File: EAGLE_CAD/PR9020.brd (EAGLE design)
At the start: 70 x 70 mm, 73 parts

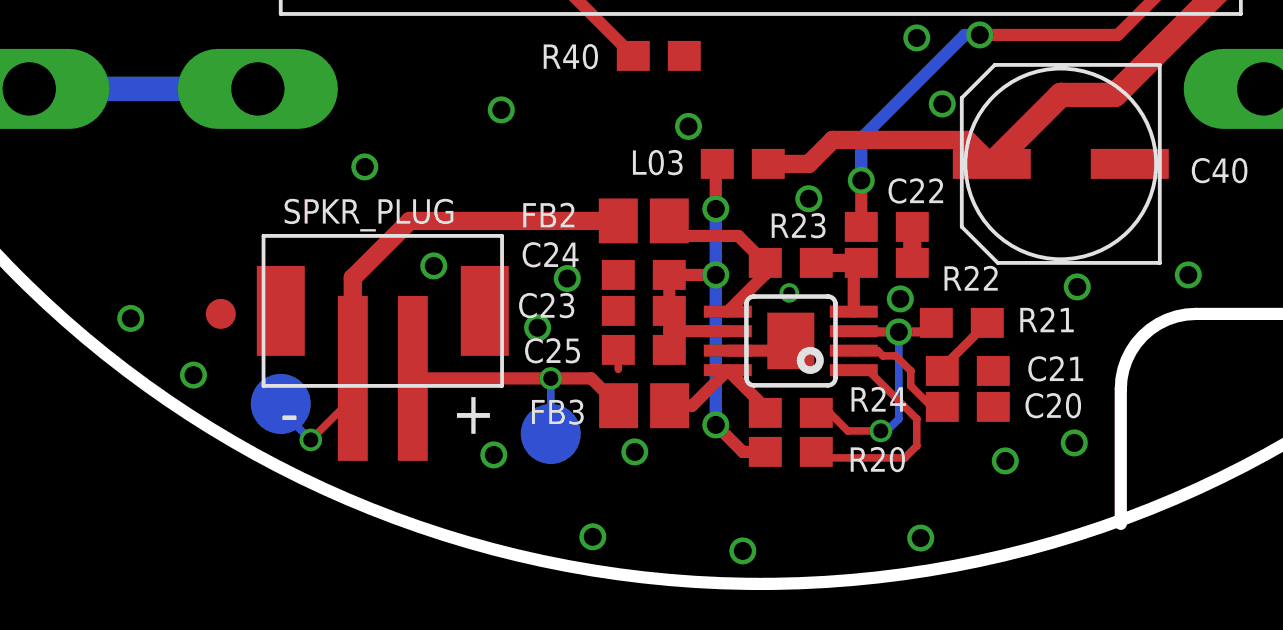
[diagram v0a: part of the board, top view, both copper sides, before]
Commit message: PR9020 Gerbers
PR9020 Gerbers, organized folders
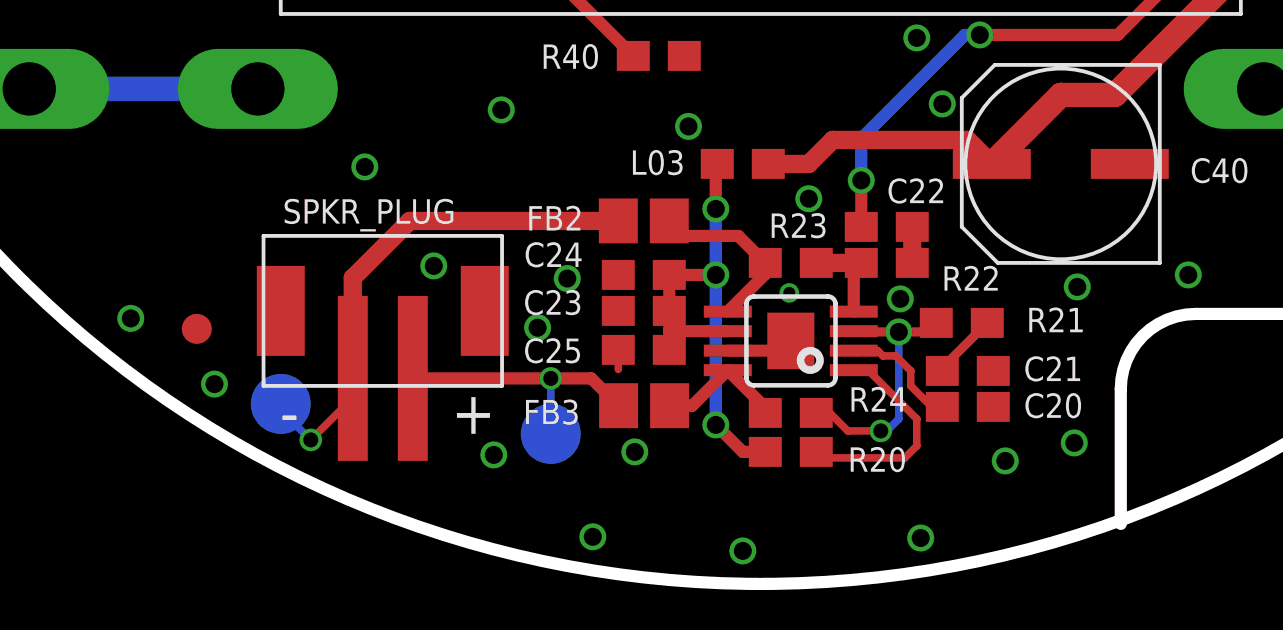
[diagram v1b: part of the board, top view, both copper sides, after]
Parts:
- moved MARK1 0.94 mm to (16.2, 8.50)
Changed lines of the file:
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@@
 <rectangle x1="35.3949" y1="12.6365" x2="35.4711" y2="12.6619" layer="26" rot="R180"/>
 <rectangle x1="35.4203" y1="12.6619" x2="35.5981" y2="12.6873" layer="26" rot="R180"/>
-<text x="64" y="35" size="0.8128" layer="26" font="vector" ratio="18" rot="MR270" align="center">PR9020
+<text x="64" y="35" size="0.8128" layer="26" font="vector" ratio="22" rot="MR270" align="center">PR9020
 Born + tuned in Brooklyn
 http://thepublicrad.io</text>
@@
 </element>
 <element name="R21" library="PR_Parts_Library" package="0603_CPL" value="12K" x="41.7" y="8.7" smashed="yes" rot="R180">
-<attribute name="NAME" x="43.551" y="8.389" size="0.8128" layer="25" font="vector" ratio="16"/>
+<attribute name="NAME" x="43.851" y="8.389" size="0.8128" layer="25" font="vector" ratio="16"/>
 <attribute name="VALUE" x="42.589" y="10.732" size="1.27" layer="27" rot="R180"/>
 <attribute name="MFG_PN" value="RC0603FR-0712KL" x="41.7" y="8.7" size="1.778" layer="27" rot="R180" display="off"/>
@@
 </element>
 <element name="C21" library="PR_Parts_Library" package="0603_CPL" value=".22uF" x="41.9" y="7.1" smashed="yes" rot="R180">
-<attribute name="NAME" x="43.861" y="6.762" size="0.8128" layer="25" font="vector" ratio="16"/>
+<attribute name="NAME" x="43.761" y="6.762" size="0.8128" layer="25" font="vector" ratio="16"/>
 <attribute name="VALUE" x="42.789" y="9.132" size="1.27" layer="27" rot="R180"/>
 <attribute name="MFG_PN" value="C1608X7R1C224K080AC" x="41.9" y="7.1" size="1.778" layer="27" rot="R180" display="off"/>
@@
 </element>
 <element name="C23" library="PR_Parts_Library" package="0603_CPL" value=".1uF" x="31.1" y="9.1" smashed="yes" rot="R180">
-<attribute name="NAME" x="26.8855" y="8.872" size="0.8128" layer="25" font="vector" ratio="16"/>
+<attribute name="NAME" x="27.0855" y="8.972" size="0.8128" layer="25" font="vector" ratio="16"/>
 <attribute name="VALUE" x="32.116" y="10.497" size="0.4064" layer="27" rot="R180"/>
 <attribute name="MFG_PN" value="CL10B104KB8SFNC" x="31.1" y="9.1" size="1.778" layer="27" rot="R180" display="off"/>
@@
 </element>
 <element name="FB2" library="PR_Parts_Library" package="0805_ADAFRUIT" value="" x="31.1" y="12.1" smashed="yes" rot="R180">
-<attribute name="NAME" x="26.985" y="11.88" size="0.8128" layer="25" font="vector" ratio="16"/>
+<attribute name="NAME" x="27.185" y="11.78" size="0.8128" layer="25" font="vector" ratio="16"/>
 <attribute name="VALUE" x="31.735" y="14.64" size="1.27" layer="27" rot="R180"/>
 <attribute name="MFG_PN" value="HI0805R800R-10" x="31.1" y="12.1" size="1.778" layer="27" rot="R180" display="off"/>
@@
 </element>
 <element name="FB3" library="PR_Parts_Library" package="0805_ADAFRUIT" value="" x="31.11" y="5.94" smashed="yes">
-<attribute name="NAME" x="27.275" y="5.32" size="0.8128" layer="25" font="vector" ratio="16"/>
+<attribute name="NAME" x="27.075" y="5.32" size="0.8128" layer="25" font="vector" ratio="16"/>
 <attribute name="VALUE" x="30.475" y="3.4" size="1.27" layer="27"/>
 <attribute name="MFG_PN" value="HI0805R800R-10" x="31.11" y="5.94" size="1.778" layer="27" display="off"/>
@@
 <attribute name="MFG_PN" value="DNP" x="39" y="68" size="1.778" layer="28" rot="MR0" display="off"/>
 </element>
-<element name="MARK1" library="PR_Parts_Library" package="FIDUCIAL_1MM" value="" x="17" y="9">
-<attribute name="MFG_PN" value="DNP" x="17" y="9" size="1.778" layer="27" display="off"/>
+<element name="MARK1" library="PR_Parts_Library" package="FIDUCIAL_1MM" value="" x="16.2" y="8.5">
+<attribute name="MFG_PN" value="DNP" x="16.2" y="8.5" size="1.778" layer="27" display="off"/>
 </element>
 <element name="MARK2" library="PR_Parts_Library" package="FIDUCIAL_1MM" value="" x="33" y="67">
@@
 </element>
 <element name="C24" library="PR_Parts_Library" package="0603_CPL" value="1uF" x="31.1" y="10.3" smashed="yes" rot="R180">
-<attribute name="NAME" x="27.005" y="10.565" size="0.8128" layer="25" font="vector" ratio="16"/>
+<attribute name="NAME" x="27.105" y="10.565" size="0.8128" layer="25" font="vector" ratio="16"/>
 <attribute name="VALUE" x="31.735" y="12.205" size="1.27" layer="27" rot="R180"/>
 <attribute name="MFG_PN" value="CL10B105KP8NNNC" x="31.1" y="10.3" size="1.778" layer="27" rot="R180" display="off"/>
@@
 <via x="46.35" y="40.8" extent="1-16" drill="0.6"/>
 <via x="43.15" y="4.1" extent="1-16" drill="0.6"/>
-<via x="16.09" y="6.96" extent="1-16" drill="0.6"/>
+<via x="16.79" y="6.66" extent="1-16" drill="0.6"/>
 <via x="21.8" y="13.9" extent="1-16" drill="0.6"/>
 <via x="28.55" y="23.6" extent="1-16" drill="0.6"/>
